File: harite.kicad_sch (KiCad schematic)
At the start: 39 parts, among them U1 RP2040_Zero

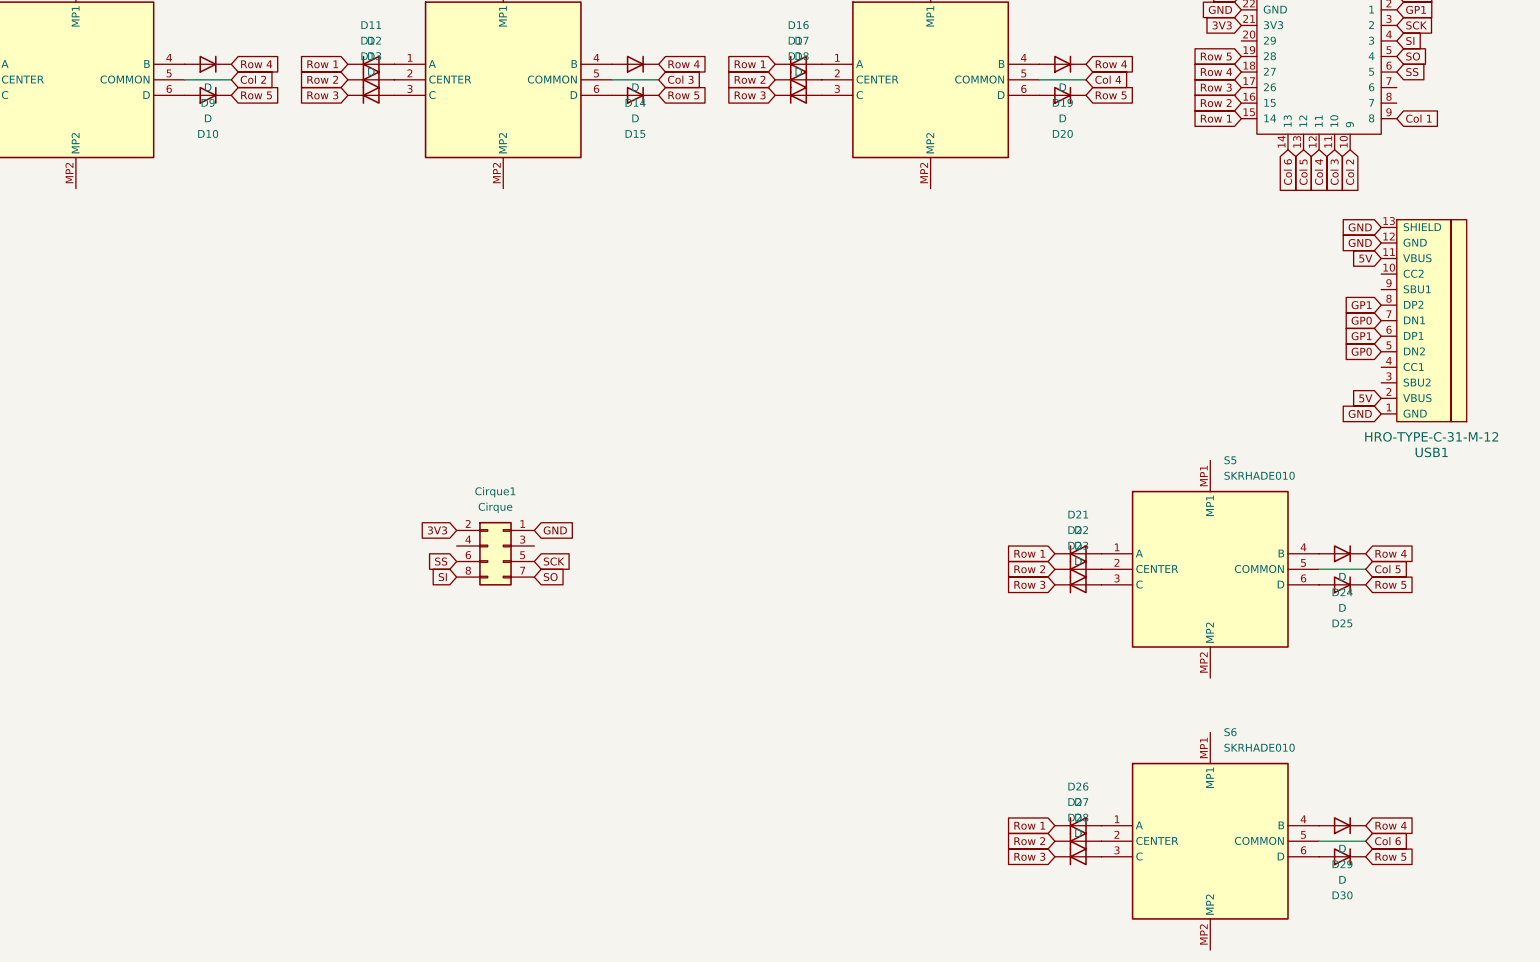
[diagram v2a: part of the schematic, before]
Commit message: Shaping
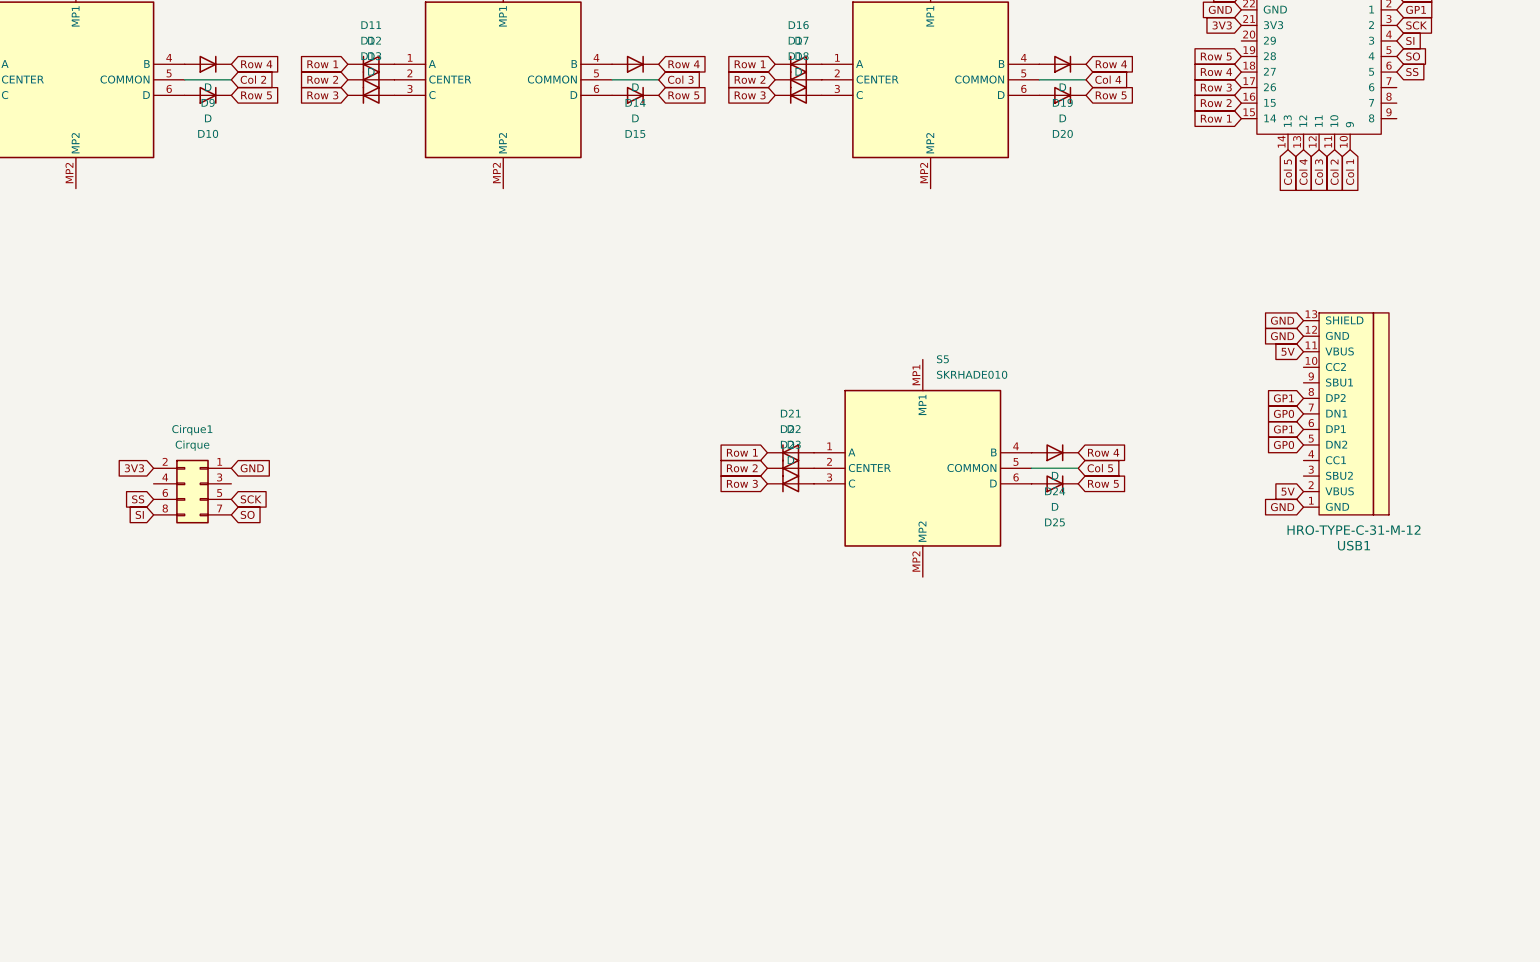
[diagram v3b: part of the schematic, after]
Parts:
- removed D26, D27, D28, D29, D30: D, ScottoKeebs_Components:Diode_SOD-123, symbol Device:D
- removed S6: SKRHADE010, footprints:SKRHADE010, symbol SKRHADE010:SKRHADE010
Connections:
- net Col 6 is gone; now on net Col 5: U1.14 (13)
- net Col 1: now also U1.10 (9); no longer U1.9 (8)
- net Col 2: now also U1.11 (10); no longer U1.10 (9)
- net Col 3: now also U1.12 (11); no longer U1.11 (10)
- net Col 4: now also U1.13 (12); no longer U1.12 (11)
- net Col 5: no longer U1.13 (12)
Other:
- moved on the sheet: Cirque1, D21, D22, D23, D24, D25, S5, USB1
